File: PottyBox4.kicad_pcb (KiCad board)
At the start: 2 copper layers, 51 x 63.5 mm, 52 parts, among them IC1 ESP32-WROVER-B, J1 Sensor 1, J10 Flush 2, J2 Touch 1, J3 Sensor 2, J4 Touch 2, J5 Qwiic, J6 24VAC, J7 DEGUG, J8 Exhaust, J9 Flush 1, K1 G3VM-61VY3, K2 G3VM-61VY3, K3 CPC1998J, Q1 MMBT3904, Q2 MMBT3904, SW1 BOOT, SW2 RESET, U1 OKI-78SR-3.3/1.5-W36H-C, U2 Adafruit_CP2104_Breakout

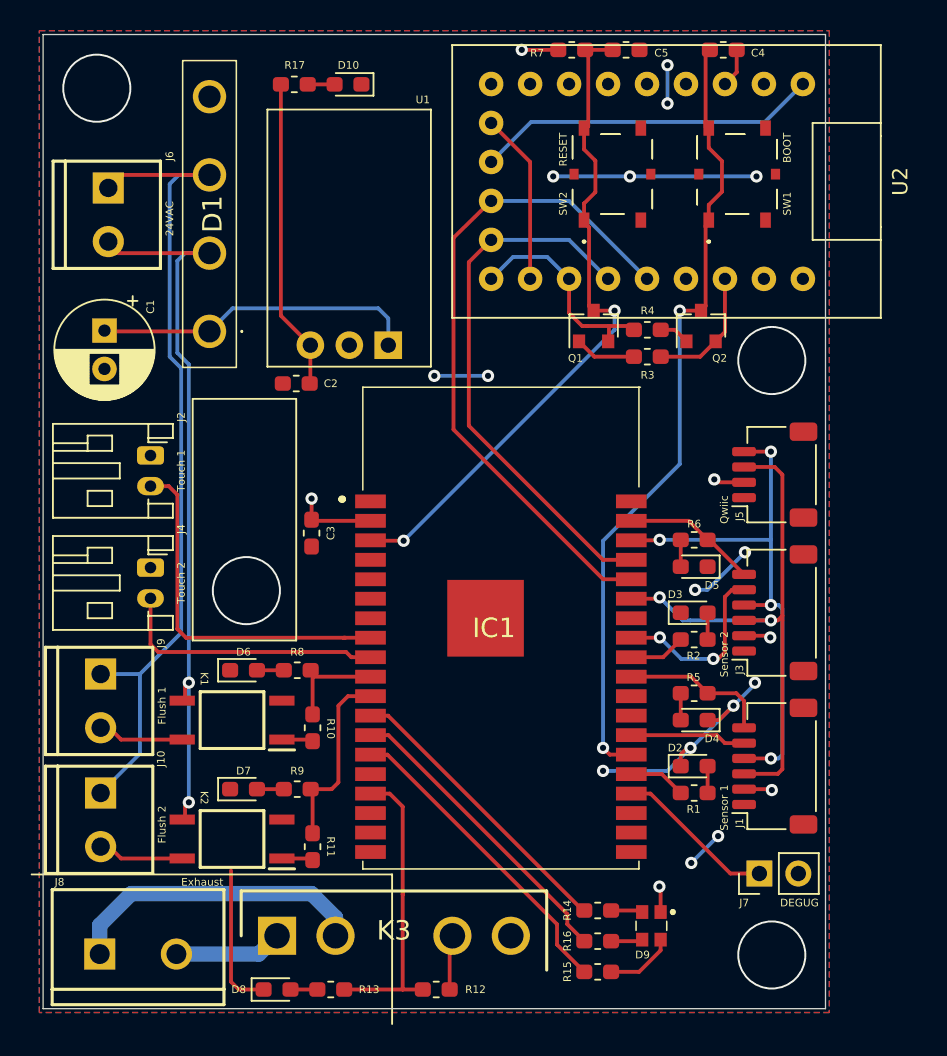
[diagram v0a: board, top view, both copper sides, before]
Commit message: Final touches
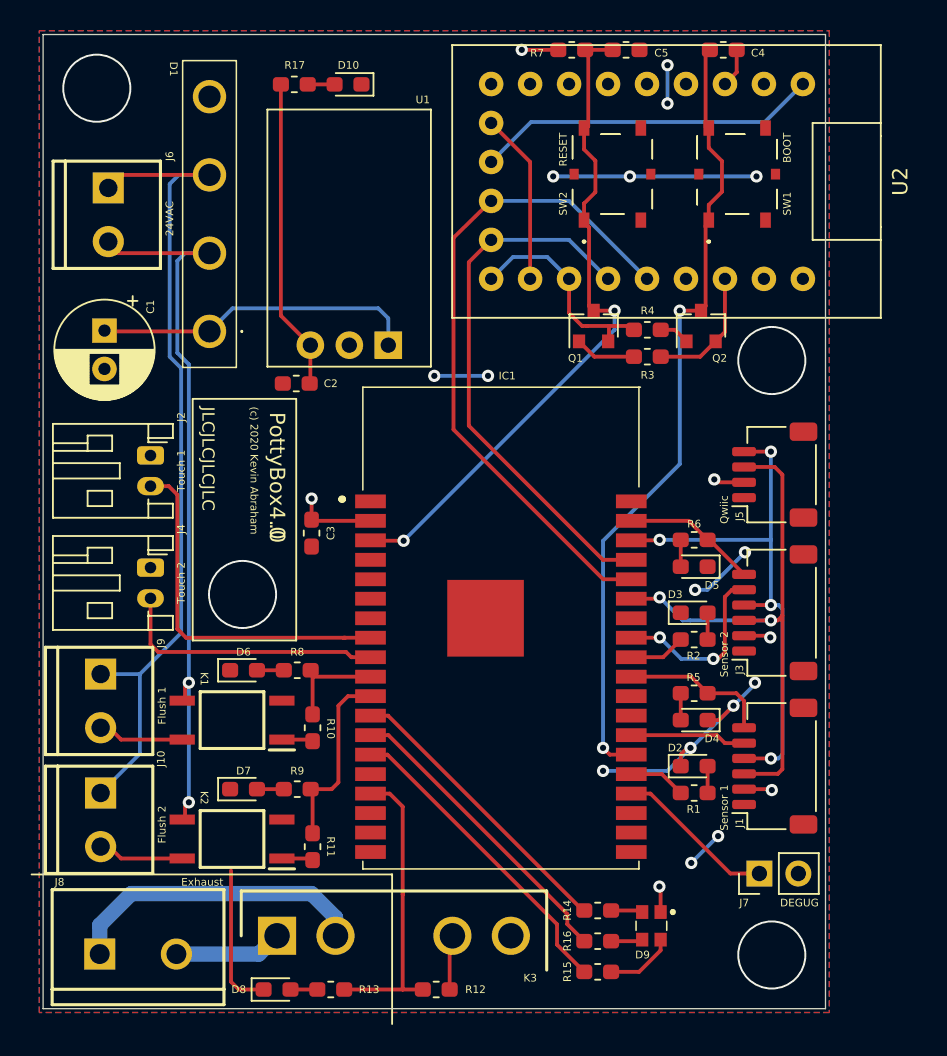
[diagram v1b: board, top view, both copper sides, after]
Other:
- board text added: "(c) 2020 Kevin Abraham"
- board text added: ".0"
- board text added: "4.0"
- board text added: "JLCJLCJLCJLC"
- board text added: "PottyBox"
